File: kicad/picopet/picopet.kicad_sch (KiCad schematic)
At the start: 59 parts, among them J1 USB_C_Receptacle_USB2.0_14P, J2 MicroJST 1.25mm female, J3 CR1220 Holder, J4 ST7735 LCD, M1 Motor_DC, Q1 SS8050, SW1 PWR, SW2 BOOTSEL, SW4 Btn0, SW5 Btn1, SW6 Btn2, SW7 Btn3, U1 RP2040, U2 MCP73831-2-OT, U3 S-T111B33MC-OGSTFU, U4 DS3231MZ, U6 AT24CS32-SSHM, U7 W25Q128JVS, Y1 ABLS-12.000MHZ-B4-T

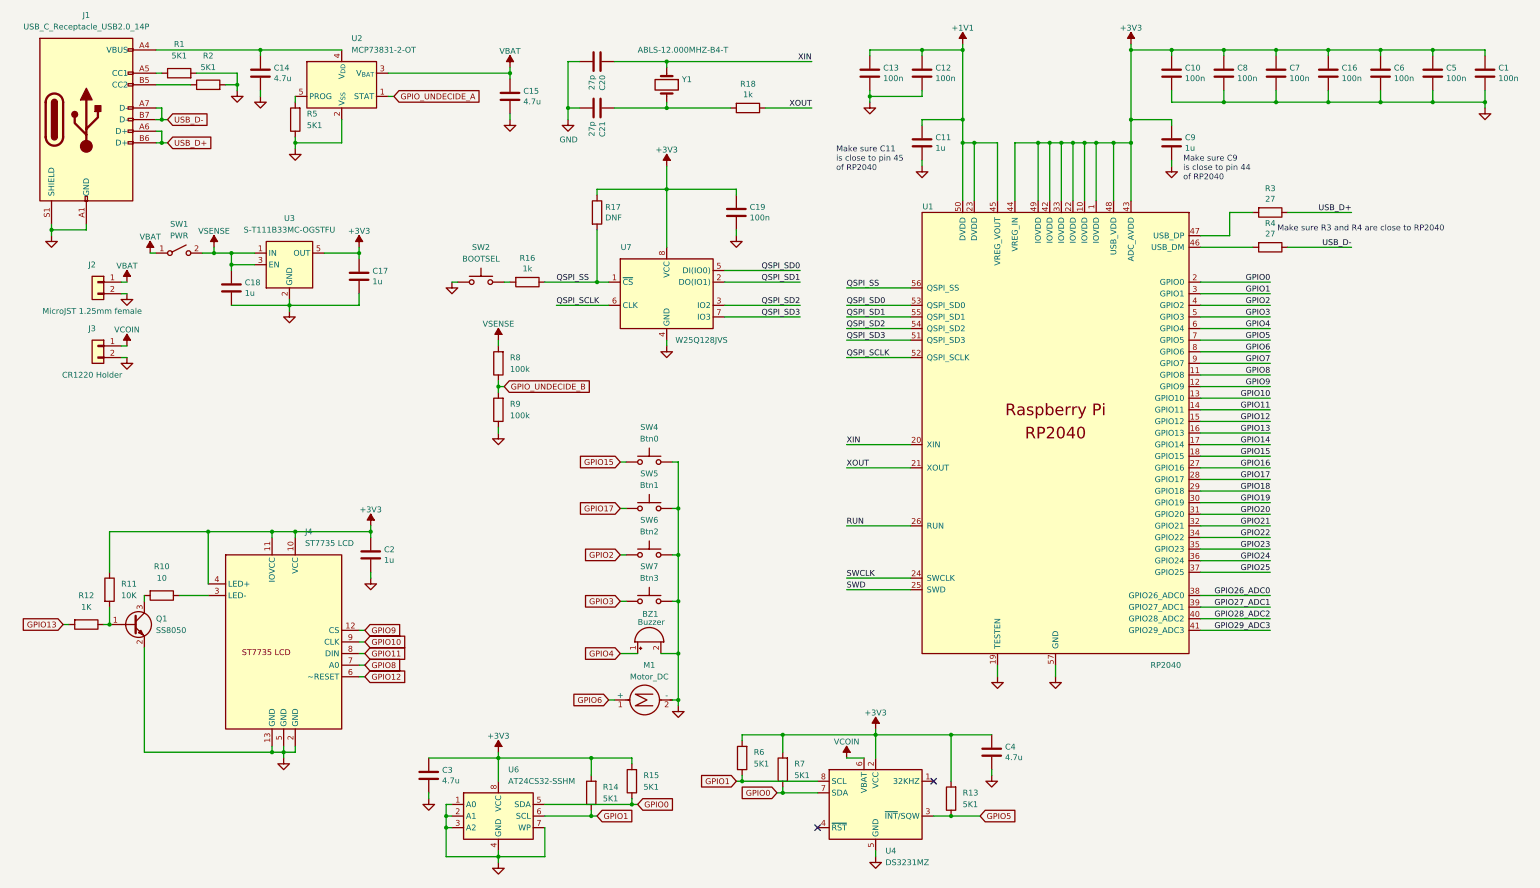
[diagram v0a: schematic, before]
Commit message: Redesigning pcb
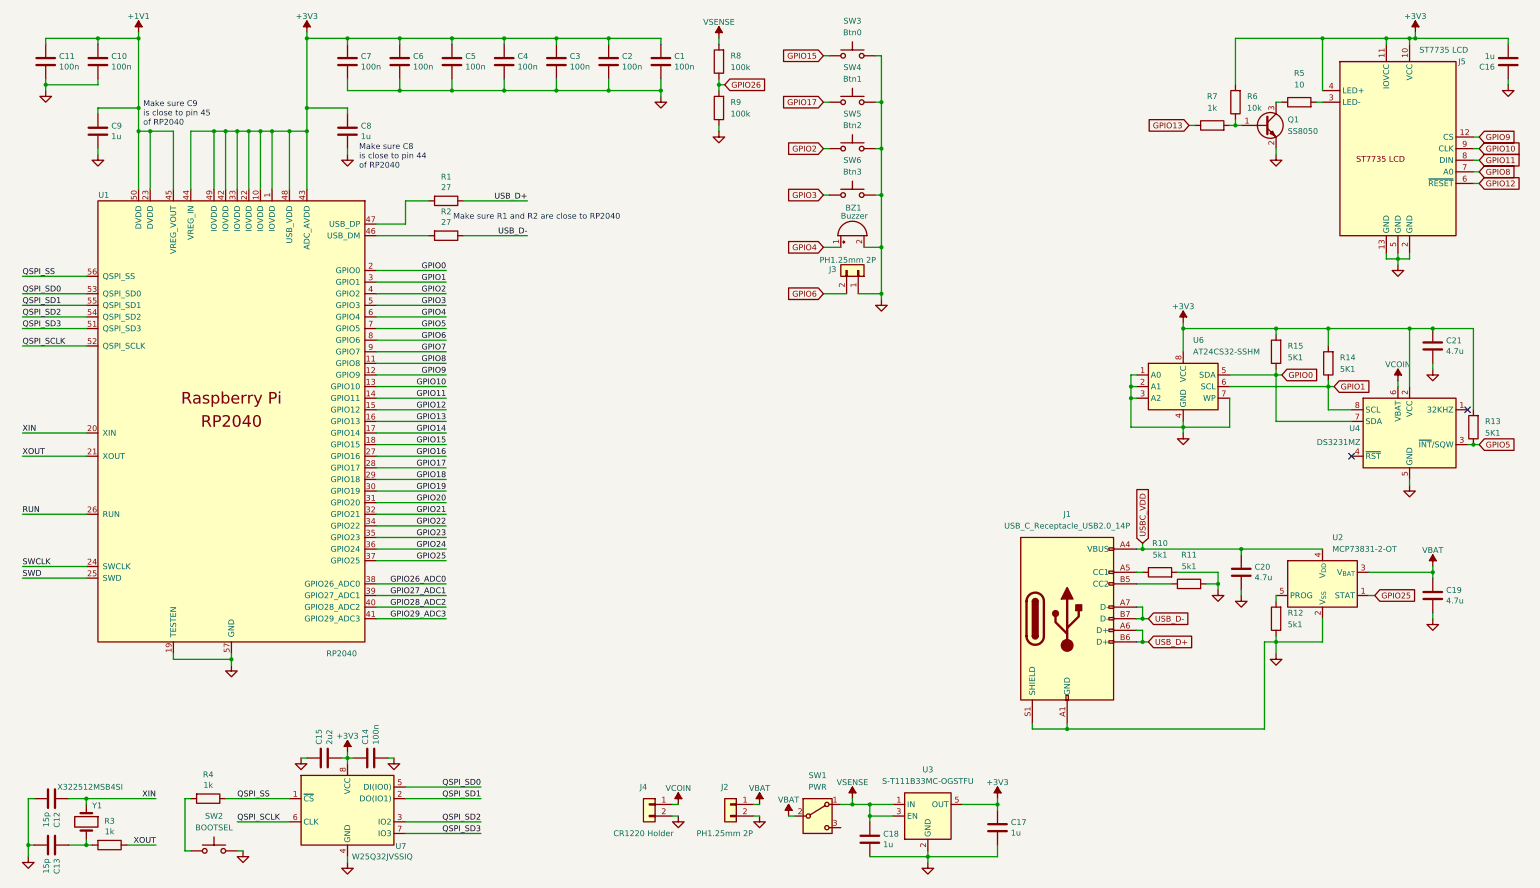
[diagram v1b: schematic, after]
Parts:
- removed C2: 1u, Capacitor_SMD:C_0805_2012Metric, symbol Device:C
- removed C3, C4: 4.7u, Capacitor_SMD:C_0805_2012Metric, symbol Device:C
- removed J4: ST7735 LCD, custom:ST7735_P0.8mm, symbol custom:ST7735
- removed M1: Motor_DC, Connector_JST:JST_GH_SM02B-GHS-TB_1x02-1MP_P1.25mm_Horizontal, symbol Motor:Motor_DC
- removed R1, R2: 5K1, Resistor_SMD:R_0402_1005Metric, symbol Device:R
- removed R12: 1K, Resistor_SMD:R_0402_1005Metric, symbol Device:R
- removed R17: DNF, Resistor_SMD:R_0402_1005Metric, symbol Device:R
- removed SW1: PWR, Button_Switch_THT:SW_Slide_SPDT_Angled_CK_OS102011MA1Q, symbol Switch:SW_SPST
- added C15: 2u2, Capacitor_SMD:C_0402_1005Metric, symbol Device:C
- added C16: 1u, Capacitor_SMD:C_0402_1005Metric, symbol Device:C
- added C21: 4.7u, Capacitor_SMD:C_0805_2012Metric, symbol Device:C
- added J4: CR1220 Holder, Battery:BatteryHolder_LINX_BAT-HLD-012-SMT, symbol Connector_Generic:Conn_01x02
- added J5: ST7735 LCD, custom:ST7735_P0.8mm, symbol custom:ST7735
- added R5: 10, Resistor_SMD:R_0201_0603Metric, symbol Device:R
- added SW1: PWR, Button_Switch_SMD:SW_SPDT_CK_JS102011SAQN, symbol Switch:SW_SPDT
- C12: renamed from C20; value 27p -> 15p
- C13: renamed from C21; value 27p -> 15p
- J2: value MicroJST 1.25mm female -> PH1.25mm 2P
- J3: value CR1220 Holder -> PH1.25mm 2P; footprint Battery:BatteryHolder_LINX_BAT-HLD-012-SMT -> Connector_JST:JST_GH_SM02B-GHS-TB_1x02-1MP_P1.25mm_Horizontal
- R10: value 10 -> 5k1; footprint Resistor_SMD:R_0402_1005Metric -> Resistor_SMD:R_0201_0603Metric
- R11: value 10K -> 5k1; footprint Resistor_SMD:R_0402_1005Metric -> Resistor_SMD:R_0201_0603Metric
- R12: renamed from R5; value 5K1 -> 5k1; footprint Resistor_SMD:R_0402_1005Metric -> Resistor_SMD:R_0201_0603Metric
- R13, R14, R15: footprint Resistor_SMD:R_0402_1005Metric -> Resistor_SMD:R_0201_0603Metric
- R4: renamed from R16; footprint Resistor_SMD:R_0402_1005Metric -> Resistor_SMD:R_0201_0603Metric
- R6: value 5K1 -> 10k; footprint Resistor_SMD:R_0402_1005Metric -> Resistor_SMD:R_0201_0603Metric
- R7: value 5K1 -> 1k; footprint Resistor_SMD:R_0402_1005Metric -> Resistor_SMD:R_0201_0603Metric
- U7: value W25Q128JVS -> W25Q32JVSSIQ; footprint Package_SO:SOIC-8_5.3x5.3mm_P1.27mm -> Package_SO:SOIC-8-1EP_3.9x4.9mm_P1.27mm_EP2.29x3mm
- Y1: value ABLS-12.000MHZ-B4-T -> X322512MSB4SI; footprint Crystal:Crystal_SMD_HC49-SD -> Crystal:Crystal_SMD_3225-4Pin_3.2x2.5mm
- renumbered C12 to C10, C13 to C11, C19 to C14, C15 to C19, C5 to C2, C14 to C20, C6 to C3, C16 to C4, C7 to C5, C8 to C6, C10 to C7, C9 to C8, C11 to C9, R3 to R1, R4 to R2, R18 to R3, SW4 to SW3, SW5 to SW4, SW6 to SW5, SW7 to SW6
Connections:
- net GPIO_UNDECIDE_A is gone; now on net GPIO25: U2.1 (STAT)
- net +3V3: now also C15.2, C16.2, C21.1, J5.10 (VCC), J5.11 (IOVCC), J5.4 (LED+); no longer R11.1, R7.2
- net GND: now also J3.1 (Pin_1), R10.2, R11.2, SW2.2, C15.1, C16.1, C21.2, J4.2 (Pin_2), J5.13 (GND), J5.2 (GND), J5.5 (GND); no longer J3.2 (Pin_2), SW2.1
- net GPIO0: no longer R7.1
- net GPIO1: no longer R6.1
- net GPIO10: now also J5.9 (CLK)
- net GPIO11: now also J5.8 (DIN)
- net GPIO12: now also J5.6 (~{RESET})
- net GPIO13: now also R7.1
- net GPIO6: now also J3.2 (Pin_2)
- net GPIO8: now also J5.7 (A0)
- net GPIO9: now also J5.12 (CS)
- net VBAT: now also SW1.2 (B)
- net VCOIN: now also J4.1 (Pin_1); no longer J3.1 (Pin_1)
- net VSENSE: now also SW1.1 (A)
- net USBC_VDD: now reaches C20.1, J1.A4 (VBUS), J1.A9 (VBUS), J1.B4 (VBUS), J1.B9 (VBUS), U2.4 (V_{DD})
- net at Q1.1 (B): now also R6.1, R7.2; no longer R11.2
- net at R4.2: now also SW2.1; no longer SW2.2
- net at R10.1: now also J1.A5 (CC1)
- net at J1.B5 (CC2): now also R11.1
- net at Q1.3 (C): now also R5.1; no longer R10.2
- net GPIO_UNDECIDE_B renamed GPIO26
- new net: J5.3 (LED-), R5.2
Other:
- note added: "Make sure C8 is close to pin 44 of RP2040"
- note added: "Make sure C9 is close to pin 45 of RP2040"
- note added: "Make sure R1 and R2 are close to RP2040"
- note removed: "Make sure C11 is close to pin 45 of RP2040"
- note removed: "Make sure C9 is close to pin 44 of RP2040"
- note removed: "Make sure R3 and R4 are close to RP2040"
- moved on the sheet: BZ1, C1, C10, C11, C12, C13, C14, C17, C18, C19, C2, C20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

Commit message: Redesigning pcb
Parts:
- U7: footprint Package_SO:SOIC-8-1EP_3.9x4.9mm_P1.27mm_EP2.29x3mm -> Package_SO:SOIC-8_3.9x4.9mm_P1.27mm
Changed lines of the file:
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@@
 			)
 		)
-		(property "Footprint" "Package_SO:SOIC-8-1EP_3.9x4.9mm_P1.27mm_EP2.29x3mm"
+		(property "Footprint" "Package_SO:SOIC-8_3.9x4.9mm_P1.27mm"
 			(at 85.09 187.96 0)
 			(effects

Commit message: Various kicad edits
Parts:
- BZ1: footprint Buzzer_Beeper:MagneticBuzzer_CUI_CMT-8504-100-SMT -> Buzzer_Beeper:MagneticBuzzer_Kobitone_254-EMB84Q-RO
- SW1: footprint Button_Switch_SMD:SW_SPDT_CK_JS102011SAQN -> Button_Switch_THT:SW_Slide_SPDT_Angled_CK_OS102011MA1Q
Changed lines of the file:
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@@
 			)
 		)
-		(property "Footprint" "Button_Switch_SMD:SW_SPDT_CK_JS102011SAQN"
+		(property "Footprint" "Button_Switch_THT:SW_Slide_SPDT_Angled_CK_OS102011MA1Q"
 			(at 187.96 189.23 0)
 			(effects
@@
 			)
 		)
-		(property "Footprint" "Buzzer_Beeper:MagneticBuzzer_CUI_CMT-8504-100-SMT"
+		(property "Footprint" "Buzzer_Beeper:MagneticBuzzer_Kobitone_254-EMB84Q-RO"
 			(at 193.04 62.865 90)
 			(effects
